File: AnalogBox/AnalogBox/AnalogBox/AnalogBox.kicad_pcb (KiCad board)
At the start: 2 copper layers, 104.5 x 47.9 mm, 13 parts, among them J1 MTJ-889X1, J11 TBLH10V-350-08BK, J2 TBLH10V-350-08BK, J3 TBLH10V-350-08BK, J4 TBLH10V-350-02BK, J5 MTJ-889X1, J6 TBLH10V-350-08BK, J8 MTJ-889X1

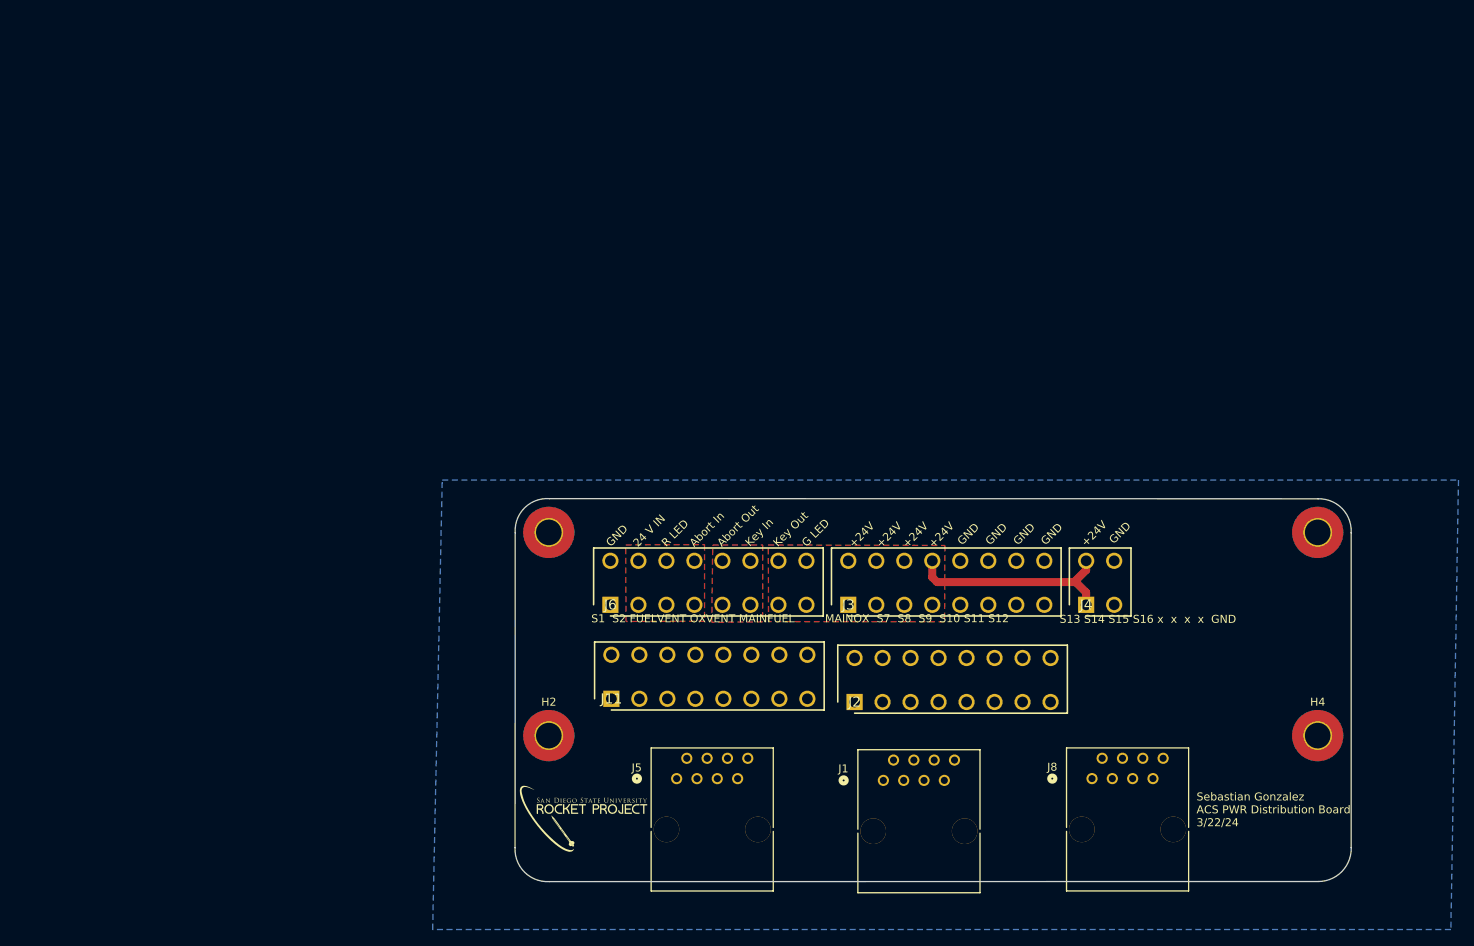
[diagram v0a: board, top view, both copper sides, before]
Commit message: Piss bot
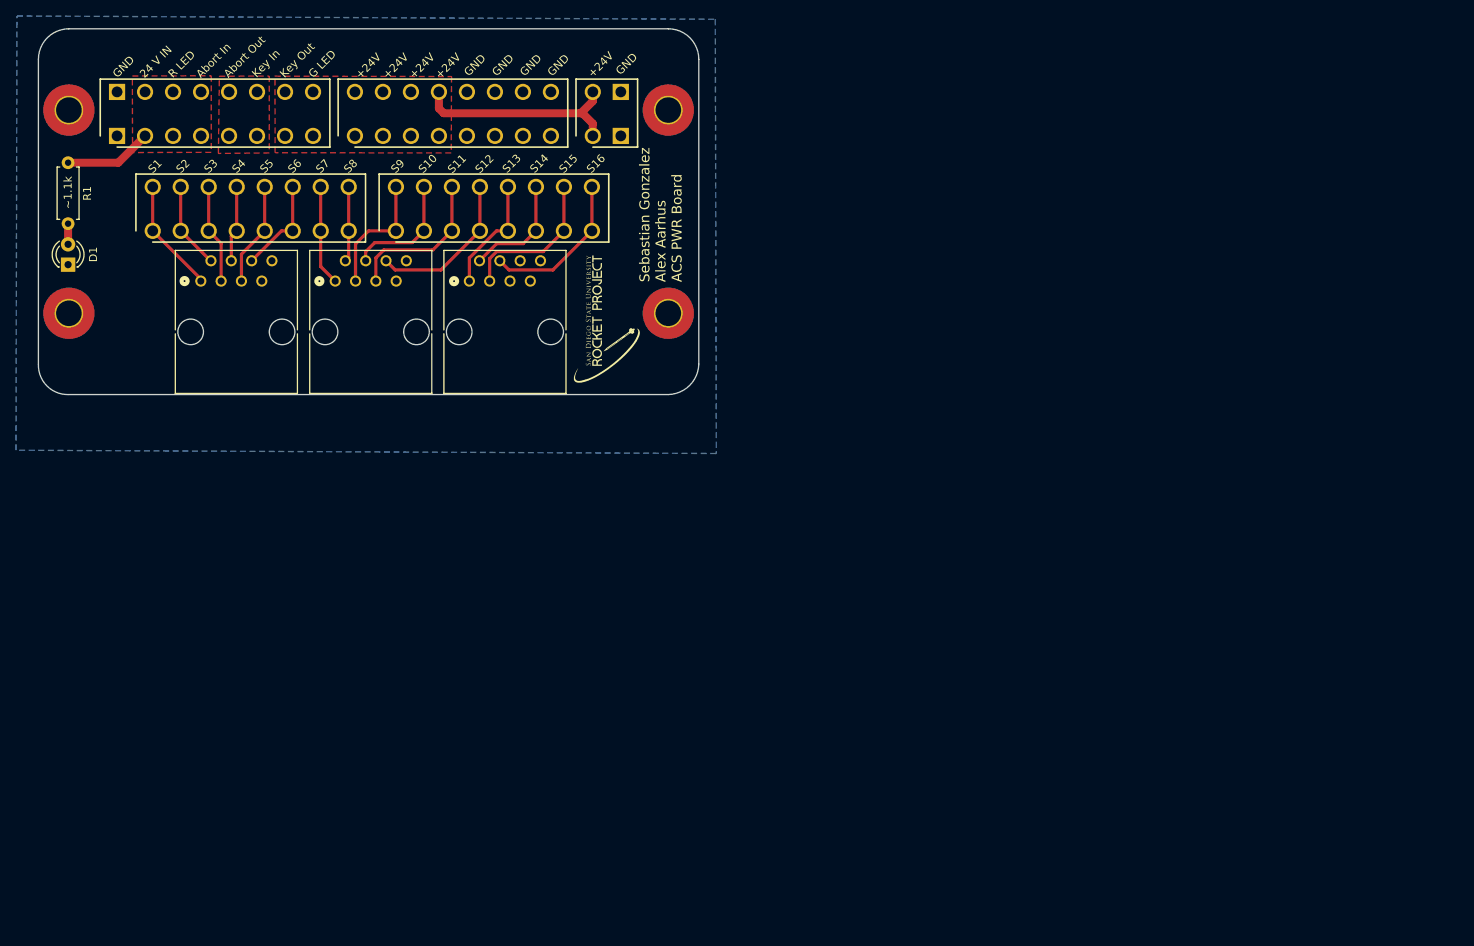
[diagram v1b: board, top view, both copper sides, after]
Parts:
- added D1: LED, LED_THT:LED_D3.0mm, F.Cu at (29.1, 54.9)
- added R1: R, Resistor_THT:R_Axial_DIN0207_L6.3mm_D2.5mm_P7.62mm_Horizontal, F.Cu at (29.1, 42.1)
- moved J8 99.6 mm to (79.3, 56.9)
- moved H4 96.8 mm to (104.1, 61.0), turned to 45 degrees
- moved H3 96.8 mm to (104.1, 35.6)
- moved J1 92.7 mm to (62.5, 56.9)
- moved J5 86.1 mm to (45.7, 56.9)
- moved J6 85.1 mm to (35.2, 38.8)
- moved J3 85.1 mm to (65.0, 38.8)
- moved J4 85.1 mm to (94.7, 38.8)
- moved J2 82.2 mm to (70.1, 50.7)
- moved J11 81.9 mm to (39.7, 50.7)
- moved H1 79.9 mm to (29.2, 35.6)
- moved H2 79.9 mm to (29.2, 61.0)
- moved G*** 62.5 mm to (96.5, 61.7), turned to 90 degrees
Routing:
- net Switch12: track 0.00 -> 19.7 mm
- net Switch16: track 0.00 -> 19.5 mm
- net Switch11: track 0.00 -> 19.3 mm
- net Switch15: track 0.00 -> 19.0 mm
- net Switch9: track 0.00 -> 15.9 mm
- net Switch10: track 0.00 -> 15.0 mm
- net Switch13: track 0.00 -> 14.6 mm
- net Switch1: track 0.00 -> 14.3 mm
- net Switch14: track 0.00 -> 14.1 mm
- net Switch5: track 0.00 -> 13.0 mm
- net Switch7: track 0.00 -> 12.5 mm
- net Switch3: track 0.00 -> 12.4 mm
- net Switch6: track 0.00 -> 12.2 mm
- net Abort In: track 0.00 -> 11.0 mm
- net Switch2: track 0.00 -> 10.8 mm
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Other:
- board size 104.5 x 47.9 mm -> 82.6 x 45.7 mm
- board text added: "S1"
- board text added: "S10"
- board text added: "S11"
- board text added: "S12"
- board text added: "S13"
- board text added: "S14"
- board text added: "S15"
- board text added: "S16"
- board text added: "S2"
- board text added: "S3"
- board text added: "S4"
- board text added: "S5"
- board text added: "S6"
- board text added: "S7"
- board text added: "S8"
- board text added: "S9"
- board text added: "Sebastian Gonzalez Alex Aarhus ACS PWR Board"
- board text added: "~1.1k"
- board text removed: "MAINOX S7 S8 S9 S10 S11 S12"
- board text removed: "S1 S2 FUELVENT OXVENT MAINFUEL"
- board text removed: "S13 S14 S15 S16 x x x x GND"
- board text removed: "Sebastian Gonzalez ACS PWR Distribution Board 3/22/24"
